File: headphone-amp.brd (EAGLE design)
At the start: 53.3 x 32 mm, 52 parts, among them IC1 OPA1612, J1 USB4125-GF-A_REVA, J3 SJ-3523-SMT-TR, J4 SJ-3523-SMT-TR, J5 SJ-3523-SMT-TR, U1 TPS65131, U2 2N7002

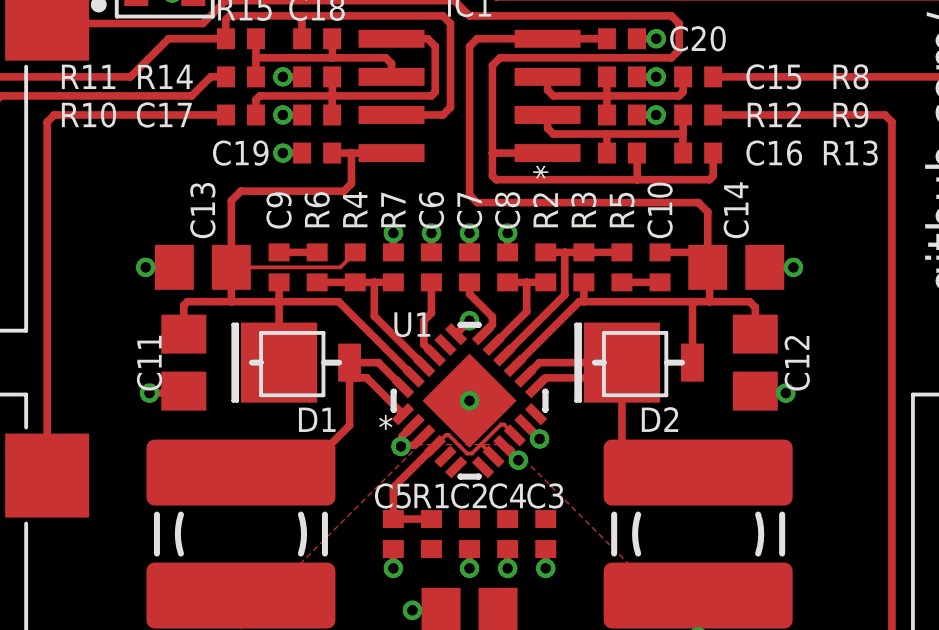
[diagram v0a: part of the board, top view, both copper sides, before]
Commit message: little routing change
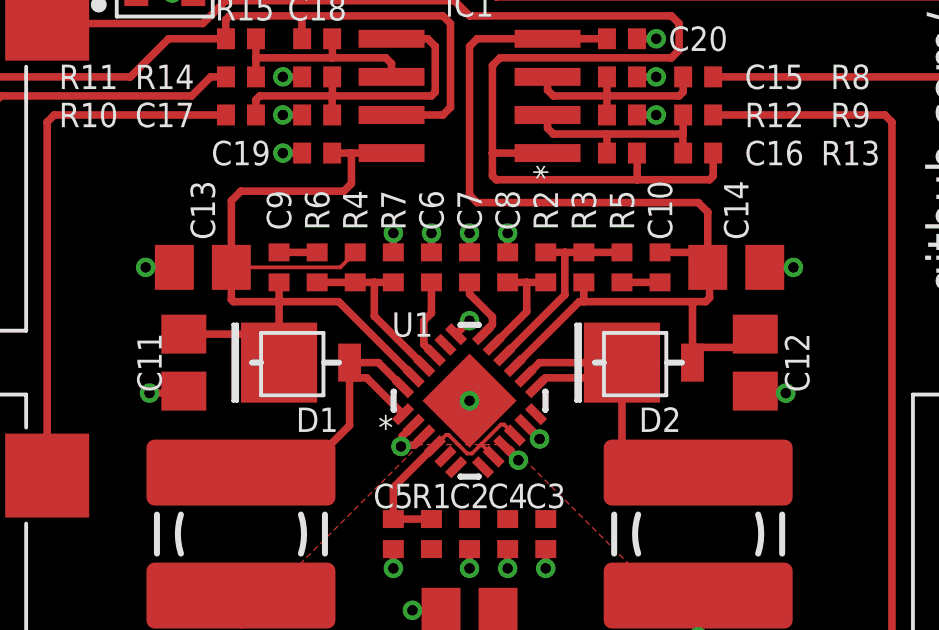
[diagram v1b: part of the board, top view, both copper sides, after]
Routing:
- net VDD: track 27.3 -> 28.0 mm
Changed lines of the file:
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@@
 <contactref element="C10" pad="1"/>
 <wire x1="28.179671875" y1="15.76111875" x2="30.325553125" y2="17.907" width="0.254" layer="1"/>
-<wire x1="34.671" y1="17.907" x2="34.671" y2="18.989" width="0.254" layer="1"/>
 <wire x1="34.671" y1="18.989" x2="34.61" y2="19.05" width="0.254" layer="1"/>
 <wire x1="30.325553125" y1="17.907" x2="30.48" y2="17.907" width="0.254" layer="1"/>
-<wire x1="30.48" y1="17.907" x2="34.163" y2="17.907" width="0.254" layer="1"/>
-<wire x1="34.163" y1="17.907" x2="34.671" y2="17.907" width="0.254" layer="1"/>
-<wire x1="34.101" y1="15.875" x2="34.101" y2="17.845" width="0.254" layer="1"/>
-<wire x1="34.101" y1="17.845" x2="34.163" y2="17.907" width="0.254" layer="1"/>
-<wire x1="36.195" y1="16.825" x2="36.195" y2="17.714" width="0.254" layer="1"/>
-<wire x1="36.195" y1="17.714" x2="36.002" y2="17.907" width="0.254" layer="1"/>
-<wire x1="36.002" y1="17.907" x2="34.671" y2="17.907" width="0.254" layer="1"/>
 <wire x1="30.48" y1="18.55" x2="30.48" y2="17.907" width="0.254" layer="1"/>
 <wire x1="33.02" y1="19.55" x2="34.11" y2="19.55" width="0.254" layer="1"/>
@@
 <wire x1="26.924" y1="21.209" x2="34.295" y2="21.209" width="0.254" layer="1"/>
 <wire x1="34.295" y1="21.209" x2="34.61" y2="20.894" width="0.254" layer="1"/>
+<wire x1="30.48" y1="17.907" x2="34.163" y2="17.907" width="0.254" layer="1"/>
+<wire x1="34.163" y1="17.907" x2="34.544" y2="17.907" width="0.254" layer="1"/>
+<wire x1="34.544" y1="17.907" x2="34.671" y2="18.034" width="0.254" layer="1"/>
+<wire x1="34.671" y1="18.034" x2="34.671" y2="18.989" width="0.254" layer="1"/>
+<wire x1="34.101" y1="15.875" x2="34.101" y2="16.383" width="0.254" layer="1"/>
+<wire x1="34.101" y1="16.383" x2="34.101" y2="17.845" width="0.254" layer="1"/>
+<wire x1="34.101" y1="17.845" x2="34.163" y2="17.907" width="0.254" layer="1"/>
+<wire x1="36.195" y1="16.825" x2="35.753" y2="16.383" width="0.254" layer="1"/>
+<wire x1="35.753" y1="16.383" x2="34.101" y2="16.383" width="0.254" layer="1"/>
 </signal>
 <signal name="VDD">
@@
 <wire x1="24.806771875" y1="15.407565625" x2="22.3073375" y2="17.907" width="0.254" layer="1"/>
 <wire x1="22.3073375" y1="17.907" x2="20.32" y2="17.907" width="0.254" layer="1"/>
-<wire x1="20.32" y1="17.907" x2="18.73" y2="17.907" width="0.254" layer="1"/>
-<wire x1="18.73" y1="17.907" x2="18.73" y2="19.05" width="0.254" layer="1"/>
-<wire x1="17.145" y1="16.825" x2="17.145" y2="17.78" width="0.254" layer="1"/>
 <wire x1="20.32" y1="18.55" x2="20.32" y2="17.907" width="0.254" layer="1"/>
-<wire x1="20.32" y1="15.875" x2="20.32" y2="17.907" width="0.254" layer="1"/>
-<wire x1="17.145" y1="17.78" x2="17.272" y2="17.907" width="0.254" layer="1"/>
-<wire x1="17.272" y1="17.907" x2="18.73" y2="17.907" width="0.254" layer="1"/>
+<wire x1="20.32" y1="15.875" x2="20.32" y2="16.51" width="0.254" layer="1"/>
+<wire x1="20.32" y1="16.51" x2="20.32" y2="17.907" width="0.254" layer="1"/>
 <wire x1="22.09" y1="22.86" x2="22.733" y2="22.86" width="0.254" layer="1"/>
 <wire x1="22.733" y1="22.86" x2="24.07" y2="22.86" width="0.254" layer="1"/>
@@
 <wire x1="22.733" y1="21.844" x2="22.733" y2="22.86" width="0.254" layer="1"/>
 <wire x1="22.479" y1="21.59" x2="22.733" y2="21.844" width="0.254" layer="1"/>
+<wire x1="17.145" y1="16.825" x2="20.005" y2="16.825" width="0.254" layer="1"/>
+<wire x1="20.005" y1="16.825" x2="20.32" y2="16.51" width="0.254" layer="1"/>
+<wire x1="18.73" y1="19.05" x2="18.73" y2="17.973" width="0.254" layer="1"/>
+<wire x1="18.73" y1="17.973" x2="18.796" y2="17.907" width="0.254" layer="1"/>
+<wire x1="18.796" y1="17.907" x2="20.32" y2="17.907" width="0.254" layer="1"/>
 </signal>
 <signal name="N$21">
